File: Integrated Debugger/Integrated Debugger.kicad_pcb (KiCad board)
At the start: 4 copper layers, 36.8 x 16.4 mm, 58 parts, among them J1 B2B GT-B0353FSV06-08B0201, J2 USB_C (PC <-> Host), J3 FPC socket 10P, J4 20021521-00010T1LF, J5 PWR, Q1 NMOS DMN2991UDA-7B, SW1 BOOT, SW2 RESET, SW3 Solar Override, SW4 Target Override, U1 USBULC6-2M6, U2 STM32F103CBUx, U3 TXB0106RGY, U4 TPS7A2633DRVR, U5 TPS22914, U6 TPS22914, Y1 8MHz

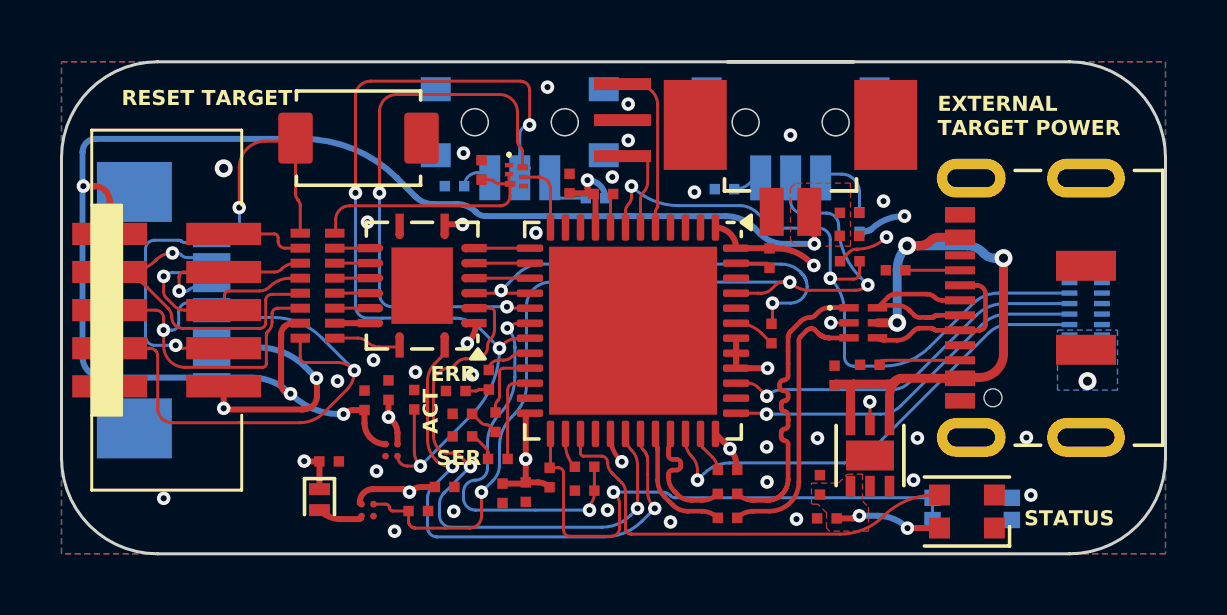
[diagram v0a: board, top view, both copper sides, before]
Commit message: PCB improvements
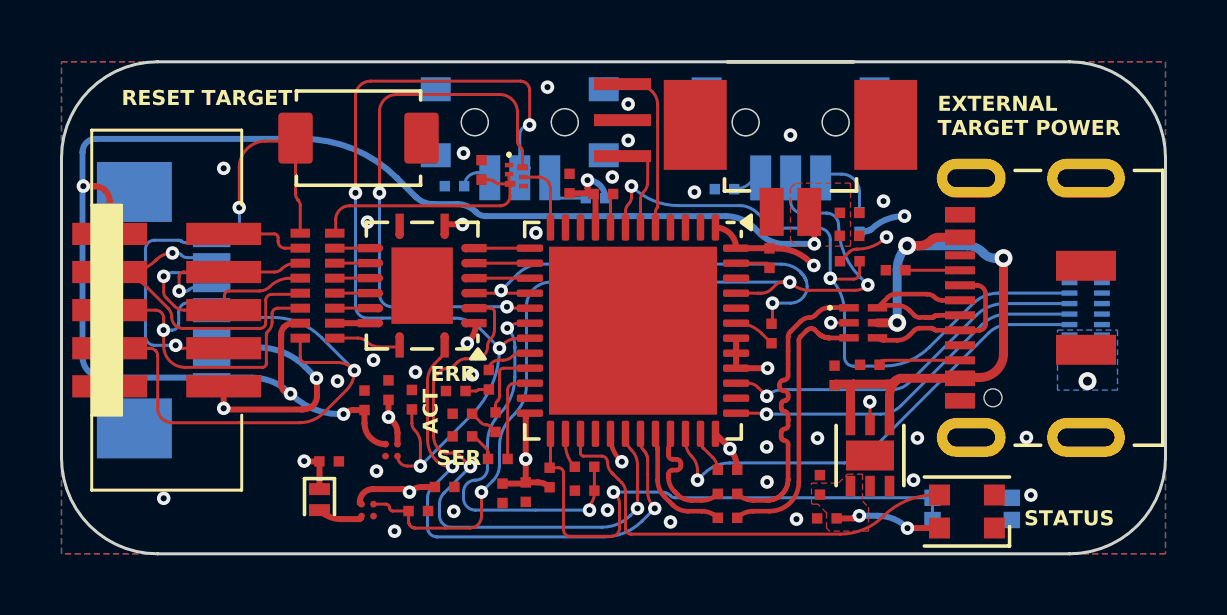
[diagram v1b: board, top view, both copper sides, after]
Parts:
- moved R14 0.08 mm to (155.4, 88.9)
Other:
- board text added: "ENIG"
- board text added: "JLC04081H-3313 JLCPCB stackup"
- board text removed: "HAL SnPb"
- board text removed: "JLC04081H-3313 JLCPCB Stackup"
